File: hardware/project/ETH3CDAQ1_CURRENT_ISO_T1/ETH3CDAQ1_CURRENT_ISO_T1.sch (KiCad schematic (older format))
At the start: 26 parts, among them J1 PC 5/2-G-7.62, J2 Conn_02x10_Odd_Even, U1 L78L15_SOT89, U2 L79L15_SOT89, U3 T60404-N4646-X400, U4 STM32F042K6Tx, U5 MCP2551-I-SN, U6 24LC08B-E/MS, U7 PCA9557PW

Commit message: PCB design
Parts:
- removed C1, C2, C3, C4: 10u/35V, symbol Device:C
- removed FB1, FB2: Ferrite_Bead, symbol Device:Ferrite_Bead
- removed R?: 120, symbol Device:R
- removed U1: L78L15_SOT89, Package_TO_SOT_SMD:SOT-89-3, symbol Regulator_Linear:L78L15_SOT89
- removed U2: L79L15_SOT89, Package_TO_SOT_SMD:SOT-89-3, symbol Regulator_Linear:L79L15_SOT89
- removed U4: STM32F042K6Tx, Package_QFP:LQFP-32_7x7mm_P0.8mm, symbol MCU_ST_STM32F0:STM32F042K6Tx
- removed U5: MCP2551-I-SN, Package_SO:SOIC-8_3.9x4.9mm_P1.27mm, symbol Interface_CAN_LIN:MCP2551-I-SN
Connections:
- wire segments 109 -> 65

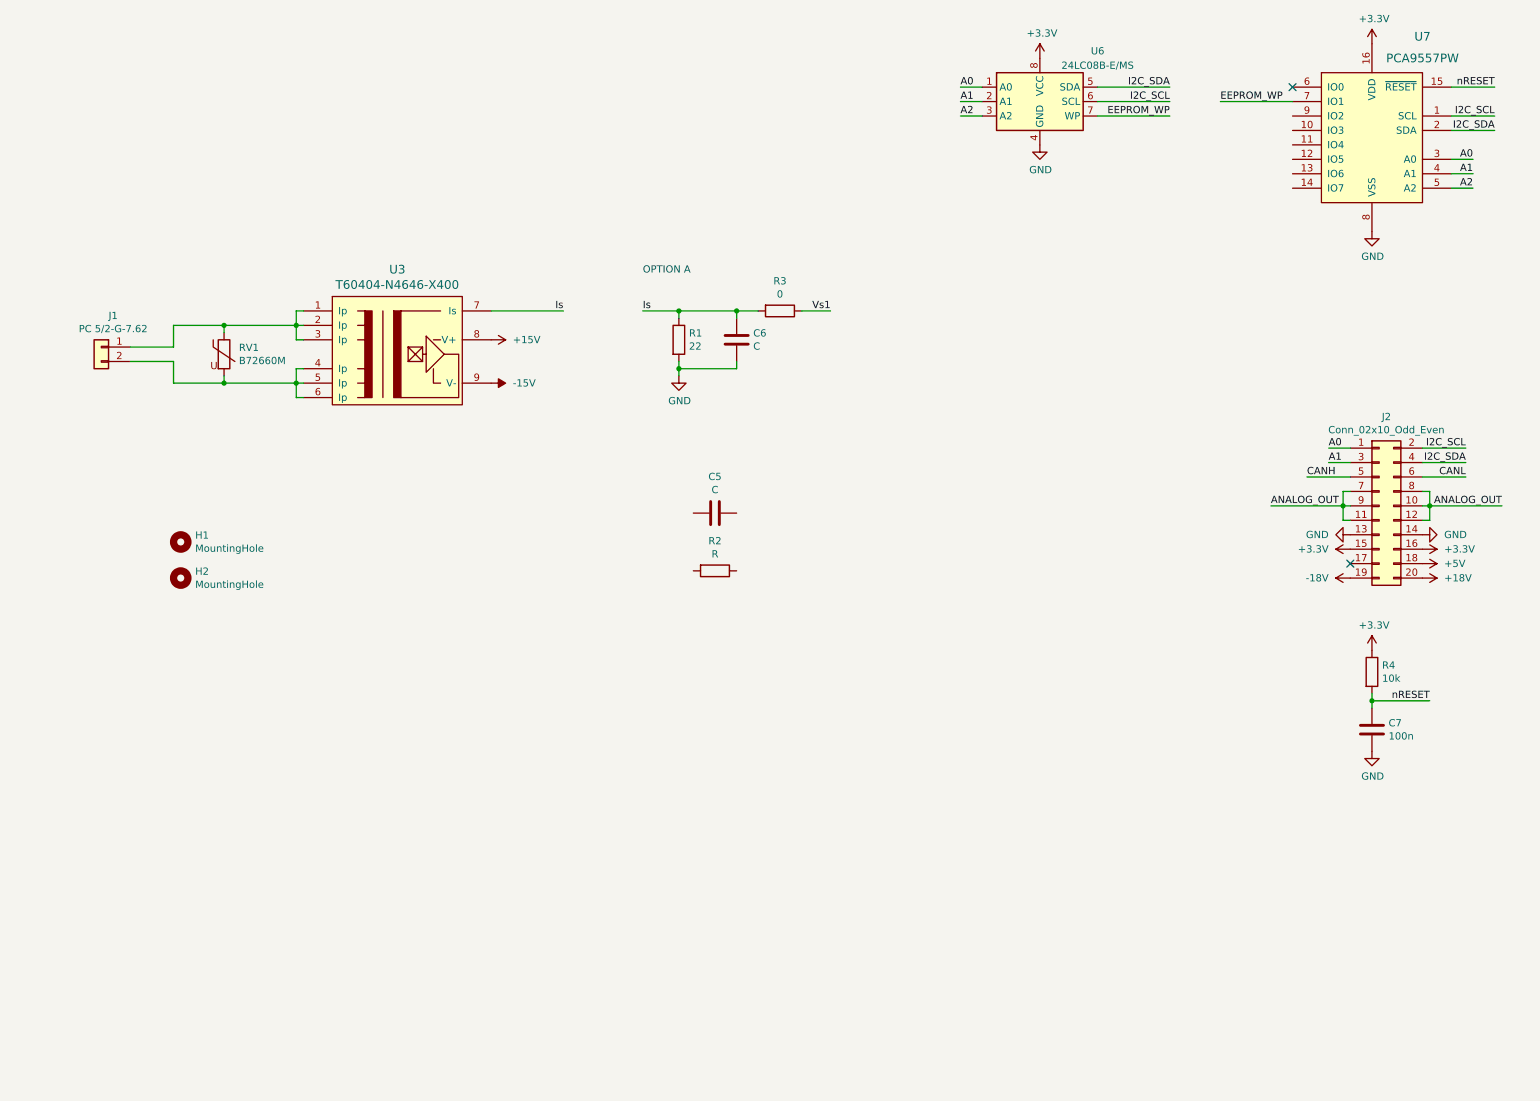
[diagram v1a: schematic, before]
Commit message: Current module development
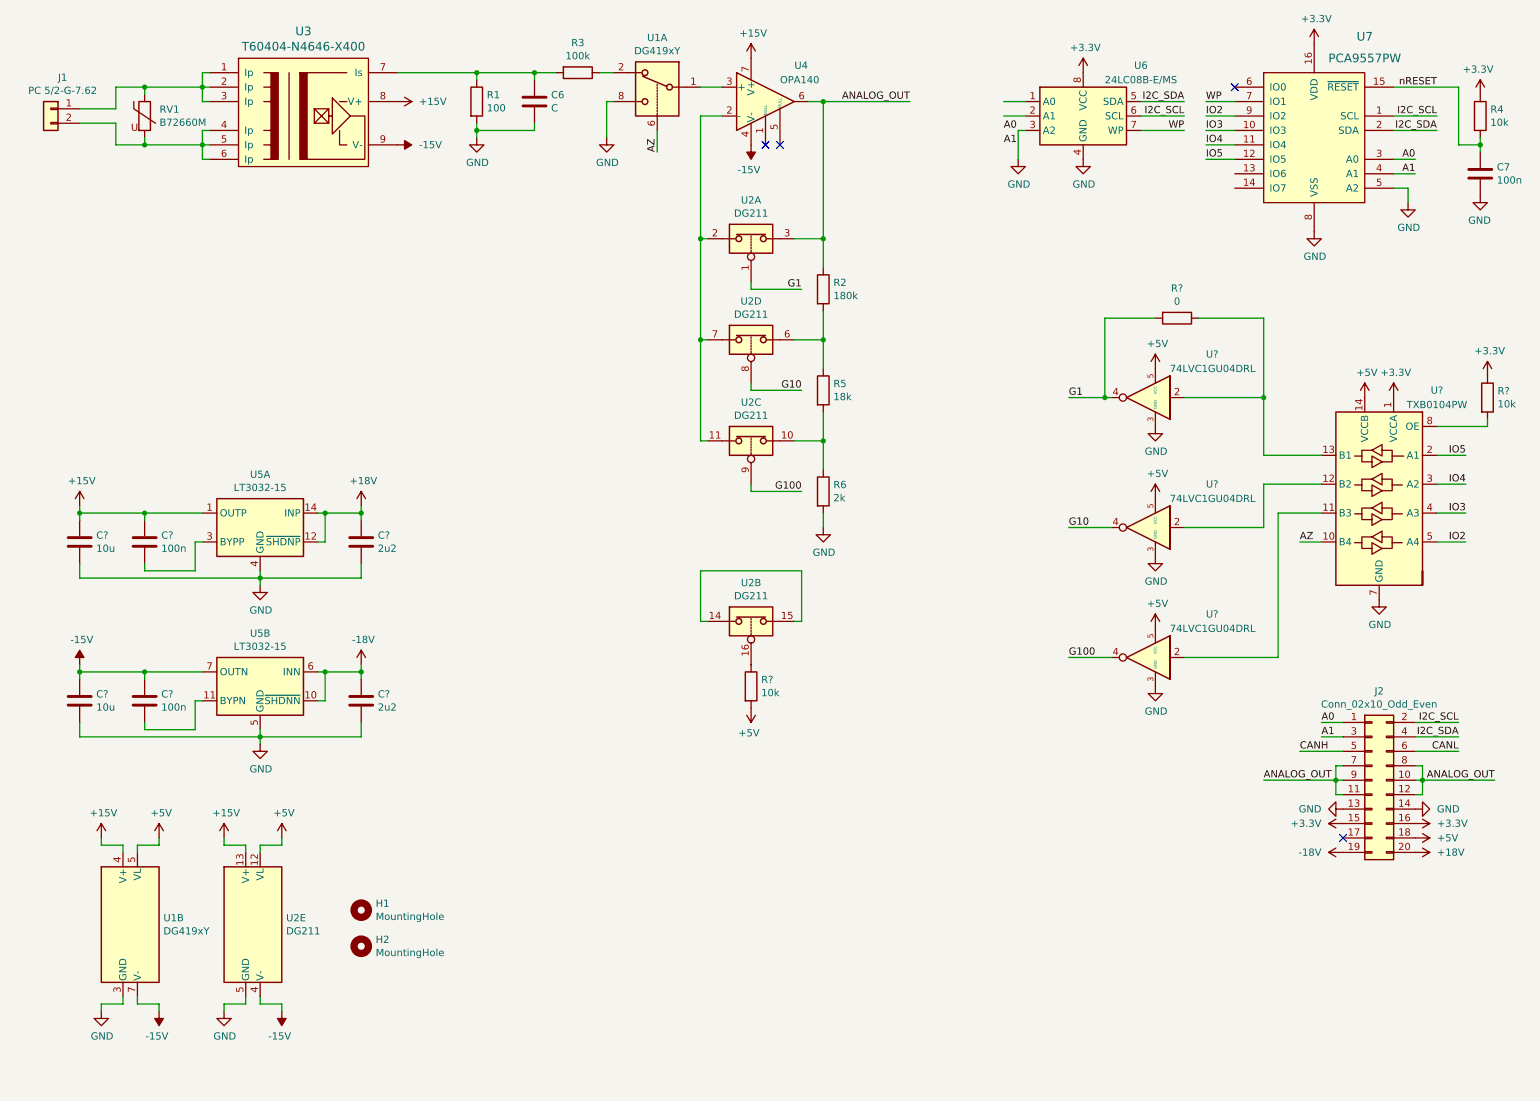
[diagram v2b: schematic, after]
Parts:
- removed C5: C, symbol Device:C
- added C? (x2): 100n, symbol Device:C
- added C? (x2): 10u, symbol Device:C
- added C? (x2): 2u2, symbol Device:C
- added R5: 18k, symbol Device:R
- added R6: 2k, symbol Device:R
- added R?: 0, symbol Device:R
- added R? (x2): 10k, symbol Device:R
- added U1: DG419xY, Package_SO:SOIC-8_3.9x4.9mm_P1.27mm, symbol Analog_Switch:DG419xY
- added U2: DG211, symbol ETH3CDAQ1:DG211
- added U4: OPA140, symbol ETH3CDAQ1:OPA140
- added U5: LT3032-15, Package_DFN_QFN:Linear_DE14MA, symbol Regulator_Linear:LT3032-15
- added U? (x3): 74LVC1GU04DRL, Package_TO_SOT_SMD:SOT-553, symbol 74xGxx:74LVC1GU04DRL
- added U?: TXB0104PW, Package_SO:TSSOP-14_4.4x5mm_P0.65mm, symbol Logic_LevelTranslator:TXB0104PW
- R1: value 22 -> 100
- R2: value R -> 180k
- R3: value 0 -> 100k
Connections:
- net A2 is gone; now on net GND: U6.3 (A2), U7.5 (A2)
- net +15V: now also C?.1, C?.1, U1.4 (V+), U2.13 (V+), U4.7 (V+), U5.1 (OUTP)
- net +18V: now also C?.1, U5.12 (~SHDNP), U5.14 (INP)
- net +3V3: now also R?.1, U?.1 (VCCA)
- net +5V: now also R?.2, U1.5 (VL), U2.12 (VL), U?.14 (VCCB), U?.5 (VCC), U?.5 (VCC), U?.5 (VCC)
- net -15V: now also C?.1, C?.1, U1.7 (V-), U2.4 (V-), U4.4 (V-), U5.7 (OUTN)
- net -18V: now also C?.1, U5.10 (~SHDNN), U5.6 (INN), U5.9 (INN)
- net A0: no longer U6.1 (A0)
- net A1: no longer U6.2 (A1)
- net ANALOG_OUT: now also R2.1, U2.3, U4.6
- net GND: now also C?.2, C?.2, C?.2, C?.2, R6.2, U1.3 (GND), U1.8, U2.5 (GND), U5.4 (GND), U5.5 (GND), U?.3 (GND), U?.3 (GND), U?.3 (GND), U?.7 (GND)
- net at R2.2: now also R5.1, U2.6
- net IO3: now reaches U7.10 (IO3)
- net IO3: now also U?.4 (A3)
- net IO4: now reaches U7.11 (IO4)
- net IO4: now also U?.3 (A2)
- net IO5: now reaches U7.12 (IO5)
- net IO5: now also U?.2 (A1)
- net IO2: now reaches U7.9 (IO2)
- net IO2: now also U?.5 (A4)
- net EEPROM_WP renamed WP
- net Is: no longer names the net of C6.1, R1.1, R3.2, U3.7 (Is)
- net Vs1: no longer names the net of R3.1
- net Vs1: now also U1.2
- new net: C?.2, U5.3 (BYPP)
- new net: C?.2, U5.11 (BYPN)
- new net: U1.1, U4.3 (+)
- new net: U2.11, U2.2, U2.7, U4.2 (-)
- new net: U2.14, U2.15
- new net: R?.1, U2.16
- new net: R5.2, R6.1, U2.10
- new net: R?.1, U?.13 (B1), U?.2
- new net: U?.12 (B2), U?.2
- new net: U?.11 (B3), U?.2
- new net: R?.2, U?.8 (OE)
- new net AZ: U1.6, U?.10 (B4)
- new net G1: R?.2, U2.1, U?.4
- new net G10: U2.8, U?.4
- new net G100: U2.9, U?.4
- no-connect marks 2 -> 4
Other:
- note removed: "OPTION A"
- moved on the sheet: C6, C7, H1, H2, J1, J2, R1, R3, R4, RV1, U3, U6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
